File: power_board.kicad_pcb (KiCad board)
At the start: 4 copper layers, 73.6 x 76.8 mm, 112 parts, among them J1 Conn_01x01, J10 Conn_01x01, J11 Conn_01x01, J12 Conn_01x01, J13 Conn_01x01, J14 Conn_01x01, J15 Conn_01x01, J16 Conn_01x01, J17 Conn_01x03, J18 Conn_01x03, J19 Conn_01x03, J2 Conn_01x01, J20 Conn_01x02, J21 Conn_01x02, J22 Conn_01x02, J23 Conn_01x01, J24 Conn_01x01, J25 Conn_01x01, J26 Conn_01x01, J3 Conn_01x01, J4 Conn_01x01, J5 Conn_01x01, J6 Conn_01x01, J7 Conn_01x01, J8 Conn_01x01, J9 Conn_01x01, Q1 IRF540S, Q2 IRF540S, Q3 IRF540S, Q4 IRF540S, U1 TPS54561, U2 TPS54561

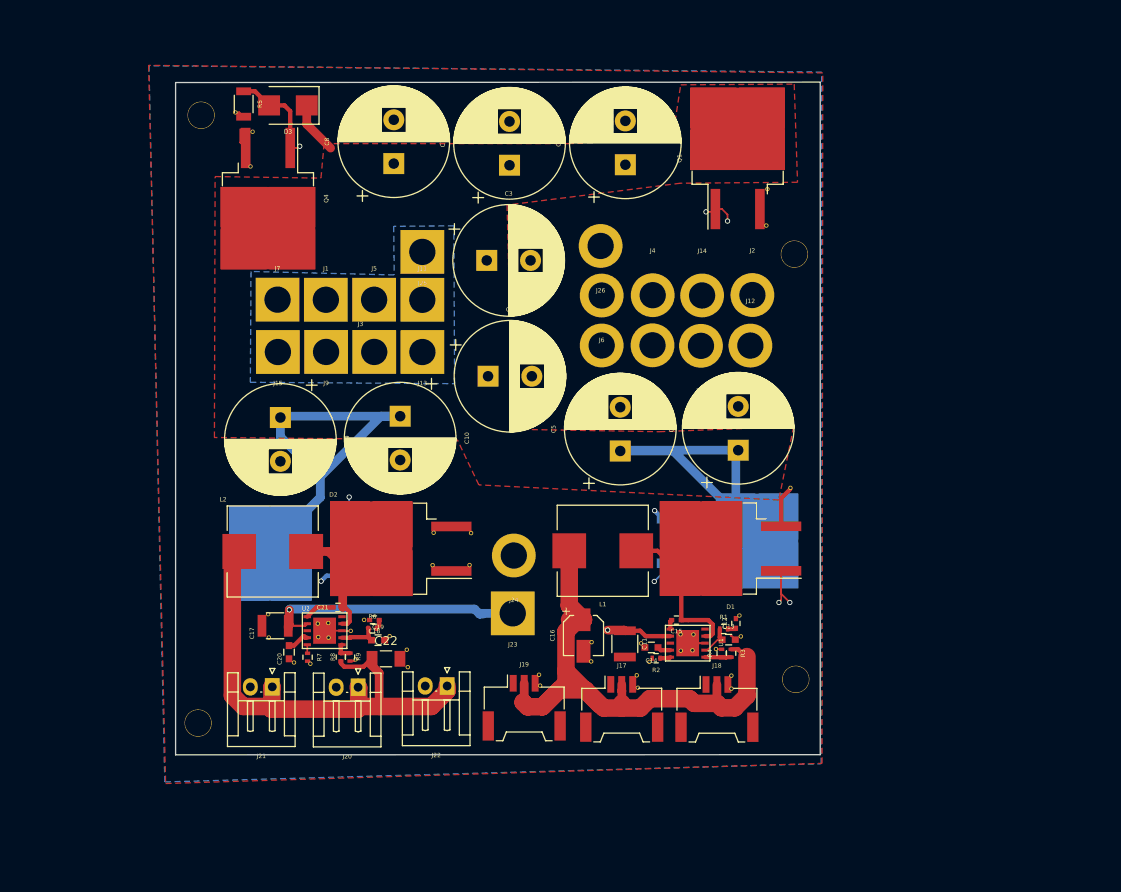
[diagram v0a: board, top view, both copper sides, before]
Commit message: now its good ?
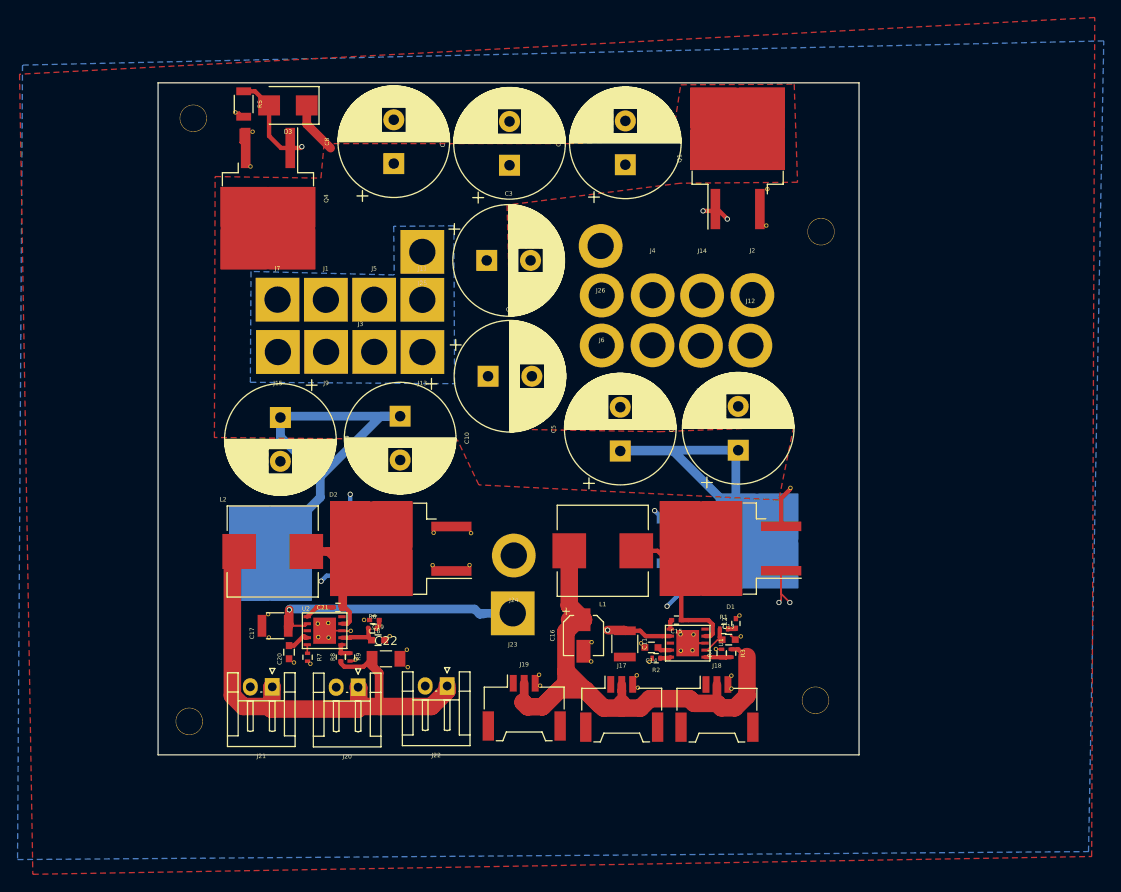
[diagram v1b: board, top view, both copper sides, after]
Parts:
- moved   3.97 mm to (179.7, 60.1)
- moved   3.28 mm to (179.0, 113.6)
- moved   1.03 mm to (107.6, 116.0)
- moved   0.96 mm to (108.0, 47.2)
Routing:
- net /Overvoltage protection/GATE: track 155.6 -> 166.7 mm
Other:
- board size 73.6 x 76.8 mm -> 80 x 76.7 mm
